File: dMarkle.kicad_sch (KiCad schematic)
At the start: 56 parts, among them SW1 SW_Choice, SW2 SW_EN, SW3 SW_RESET, U1 Pico, U2 74HC4511, U3 74HC4511, U4 74HC4511

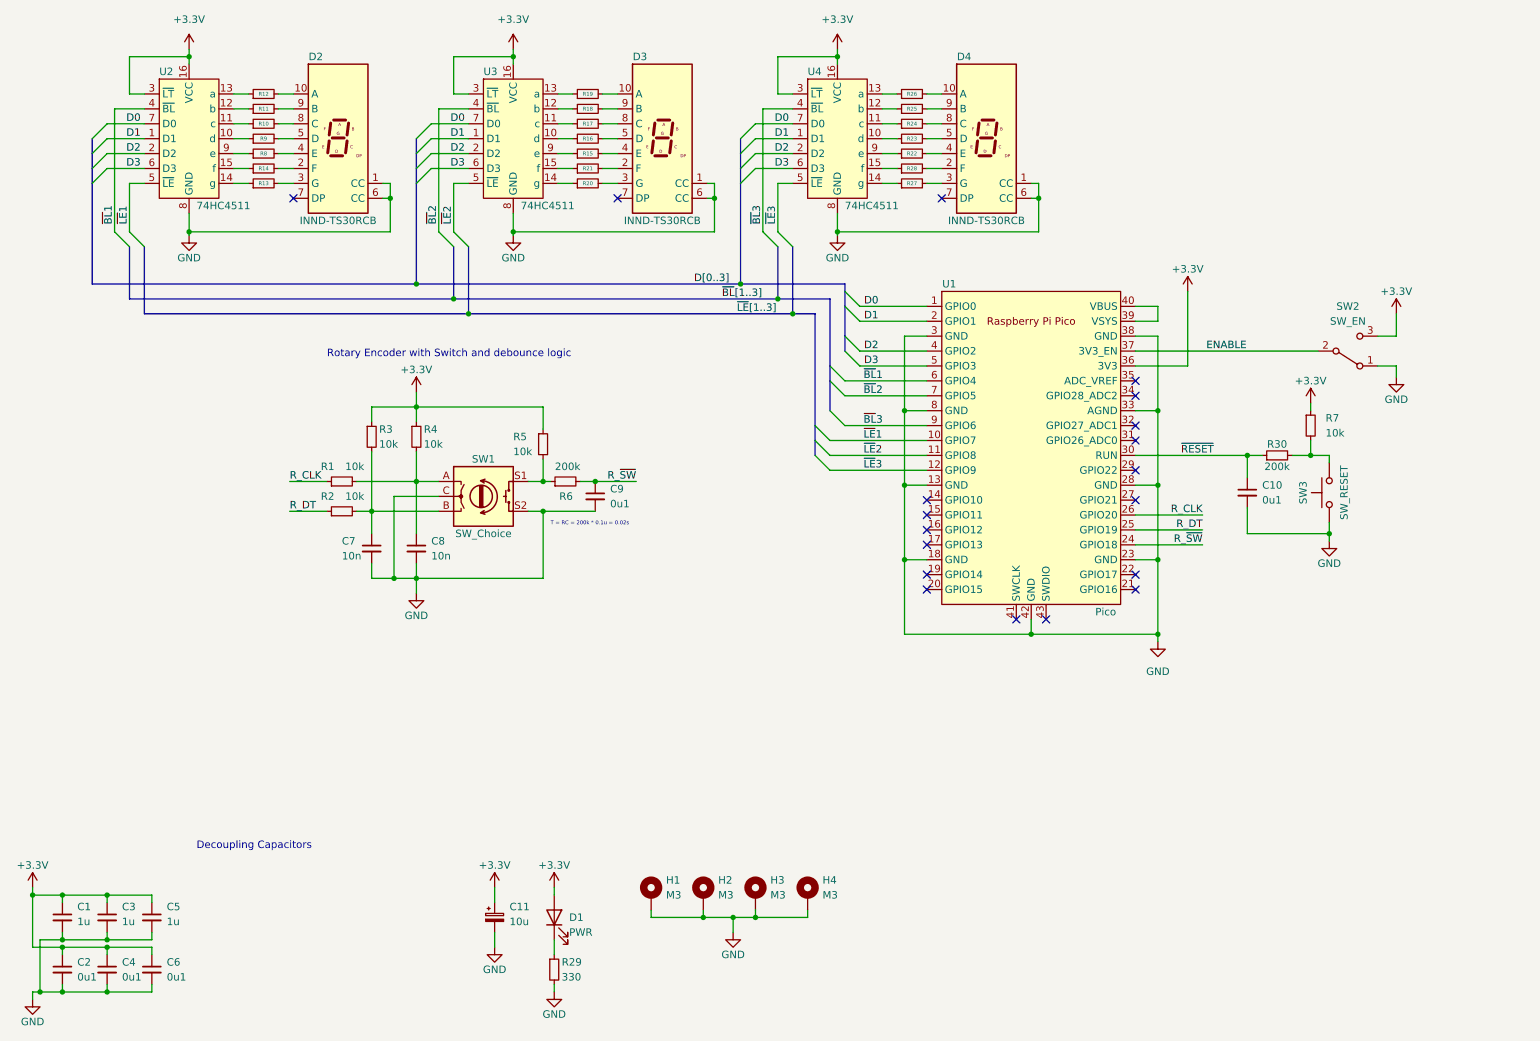
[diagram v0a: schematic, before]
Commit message: Clean up schematic and generate output for rev 0.1
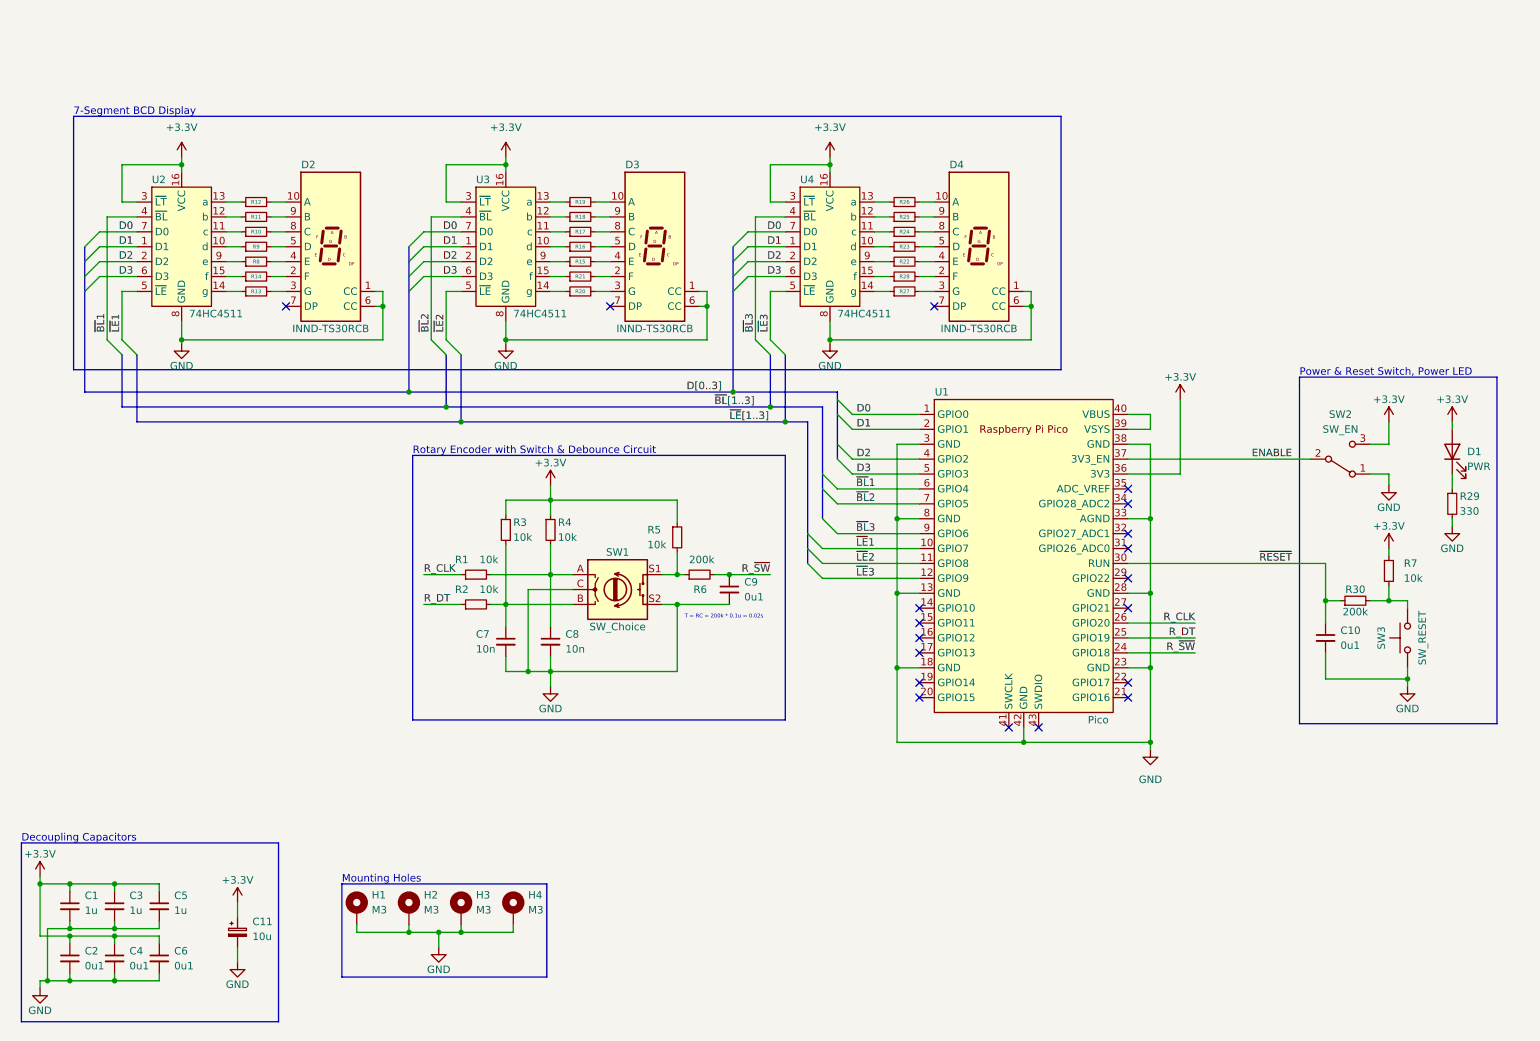
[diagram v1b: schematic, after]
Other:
- note added: "7-Segment BCD Display"
- note added: "Mounting Holes"
- note added: "Power & Reset Switch, Power LED"
- note added: "Rotary Encoder with Switch & Debounce Circuit"
- note removed: "Rotary Encoder with Switch and debounce logic"
- moved on the sheet: C1, C10, C11, C2, C3, C4, C5, C6, C7, C8, C9, D1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

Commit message: Board and parts ordered.
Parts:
- C1, C3, C5: Manufacturer (none) -> TDK Corporation; Manufacturer Part Number (none) -> FG18X5R1H105KRT06; Supplier Part Number (none) -> 445-173257-1-ND
- C10, C2, C4, C6, C9: Manufacturer (none) -> Vishay Beyschlag/Draloric/BC Components; Manufacturer Part Number (none) -> K104K15X7RF5TL2; Supplier Part Number (none) -> BC1084CT-ND
- C11: Manufacturer (none) -> Rubycon; Manufacturer Part Number (none) -> 50YXM10MEFRTA5X11; Supplier Part Number (none) -> 1189-50YXM10MEFRTA5X11CT-ND
- C7, C8: Manufacturer (none) -> Vishay Beyschlag/Draloric/BC Components; Manufacturer Part Number (none) -> K103K15X7RF5TL2; Supplier Part Number (none) -> BC1078CT-ND
- D1: Manufacturer (none) -> Würth Elektronik; Manufacturer Part Number (none) -> 151031SS04000; Supplier Part Number (none) -> 732-5005-ND
- D2, D3, D4: Manufacturer (none) -> Inolux; Manufacturer Part Number (none) -> INND-TS30RCB; Supplier Part Number (none) -> 1830-1149-ND
- R1, R2, R3, R4, R5, R7: Manufacturer (none) -> Vishay Beyschlag/Draloric/BC Components; Manufacturer Part Number (none) -> MBA02040C1002FRP00; Supplier Part Number (none) -> BC10.0KXCT-ND
- R10, R11, R12, R13, R14, R15, R16, R17, R18, R19, R20, R21, R22, R23, R24, R25, R26, R27, R28, R29, R8, R9: Manufacturer (none) -> Vishay Beyschlag/Draloric/BC Components; Manufacturer Part Number (none) -> MBA02040C3300FCT00; Supplier Part Number (none) -> BC3292CT-ND
- R30, R6: Manufacturer (none) -> Vishay Beyschlag/Draloric/BC Components; Manufacturer Part Number (none) -> MBA02040C2003FCT00; Supplier Part Number (none) -> BC3256CT-ND
- SW2: Manufacturer (none) -> C&K; Manufacturer Part Number (none) -> OS102011MA1QN1; Supplier Part Number (none) -> CKN9559-ND
- SW3: Manufacturer (none) -> E-Switch; Manufacturer Part Number (none) -> TL1105F160Q; Supplier Part Number (none) -> EG1827-ND
- U1: Manufacturer (none) -> Raspberry Pi; Manufacturer Part Number (none) -> SC0917; Supplier Part Number (none) -> 2648-SC0917-ND
- U2, U3, U4: Manufacturer (none) -> Texas Instruments; Manufacturer Part Number (none) -> CD74HC4511E; Supplier Part Number (none) -> 296-14537-5-ND
